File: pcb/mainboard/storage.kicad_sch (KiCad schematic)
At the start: 6 parts

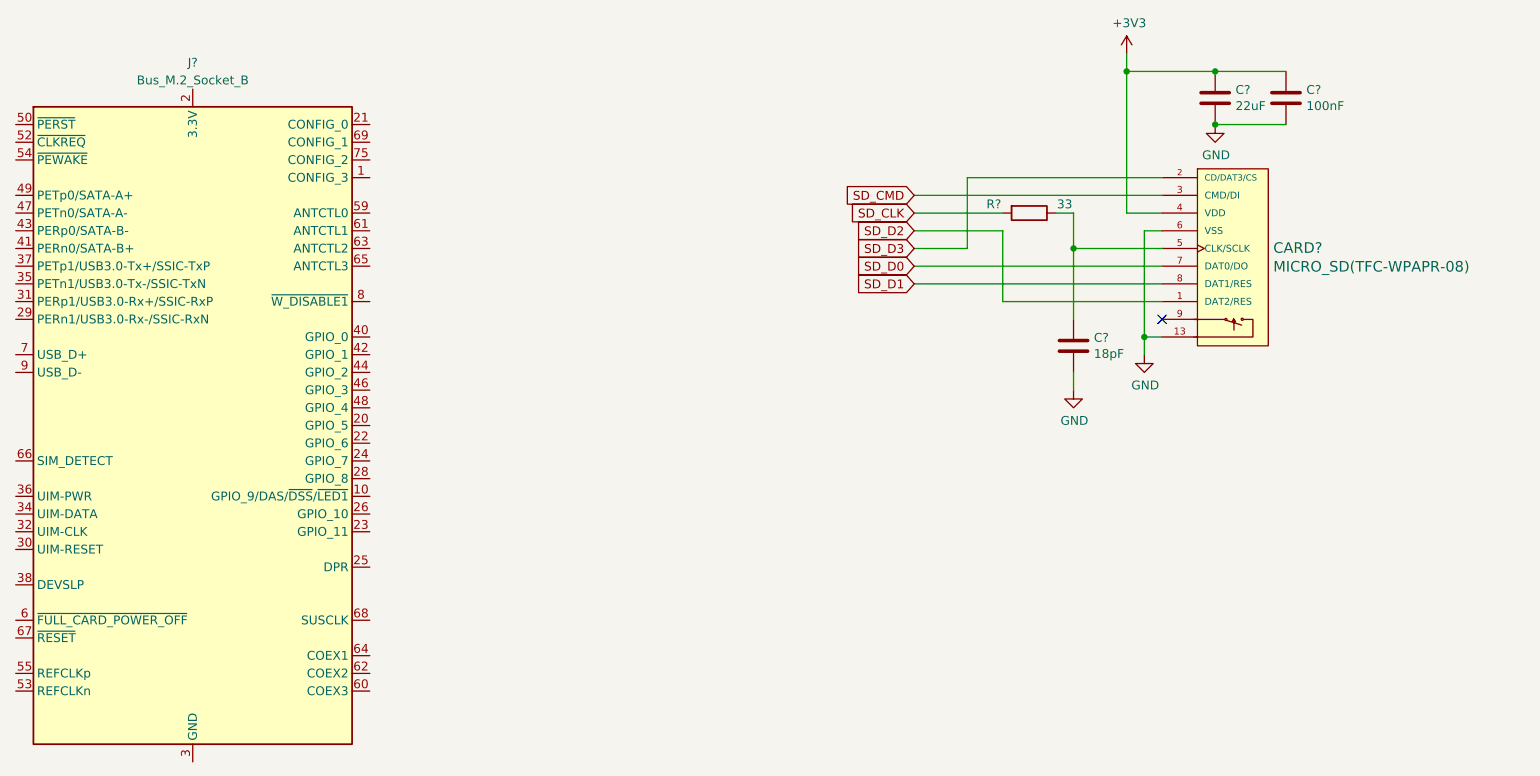
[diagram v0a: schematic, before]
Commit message: - pcb: working on r0p1 sch
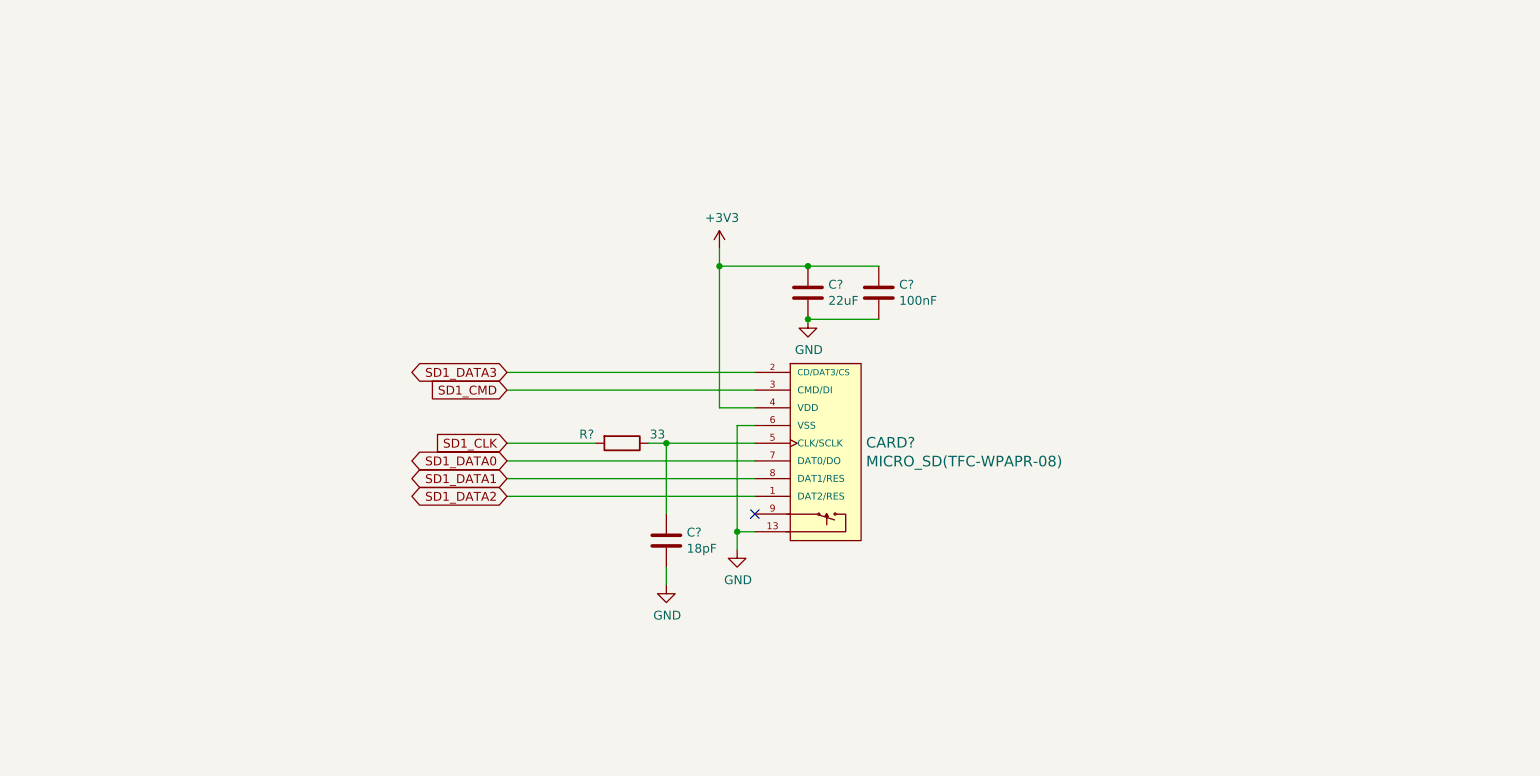
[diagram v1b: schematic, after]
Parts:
- removed J?: Bus_M.2_Socket_B, footprints:M2_BKEY, symbol Connector:Bus_M.2_Socket_B
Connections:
- net SD_CLK renamed SD1_CLK
- net SD_CMD renamed SD1_CMD
- net SD_D0 renamed SD1_DATA0
- net SD_D1 renamed SD1_DATA1
- net SD_D2 renamed SD1_DATA2
- net SD_D3 renamed SD1_DATA3
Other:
- moved on the sheet: C?, CARD?, R?
